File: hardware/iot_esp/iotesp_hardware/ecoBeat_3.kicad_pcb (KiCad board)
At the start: 2 copper layers, 67.6 x 58.6 mm, 8 parts, among them J1 Test, P1 CONN_02X05, U1 WeMos_mini

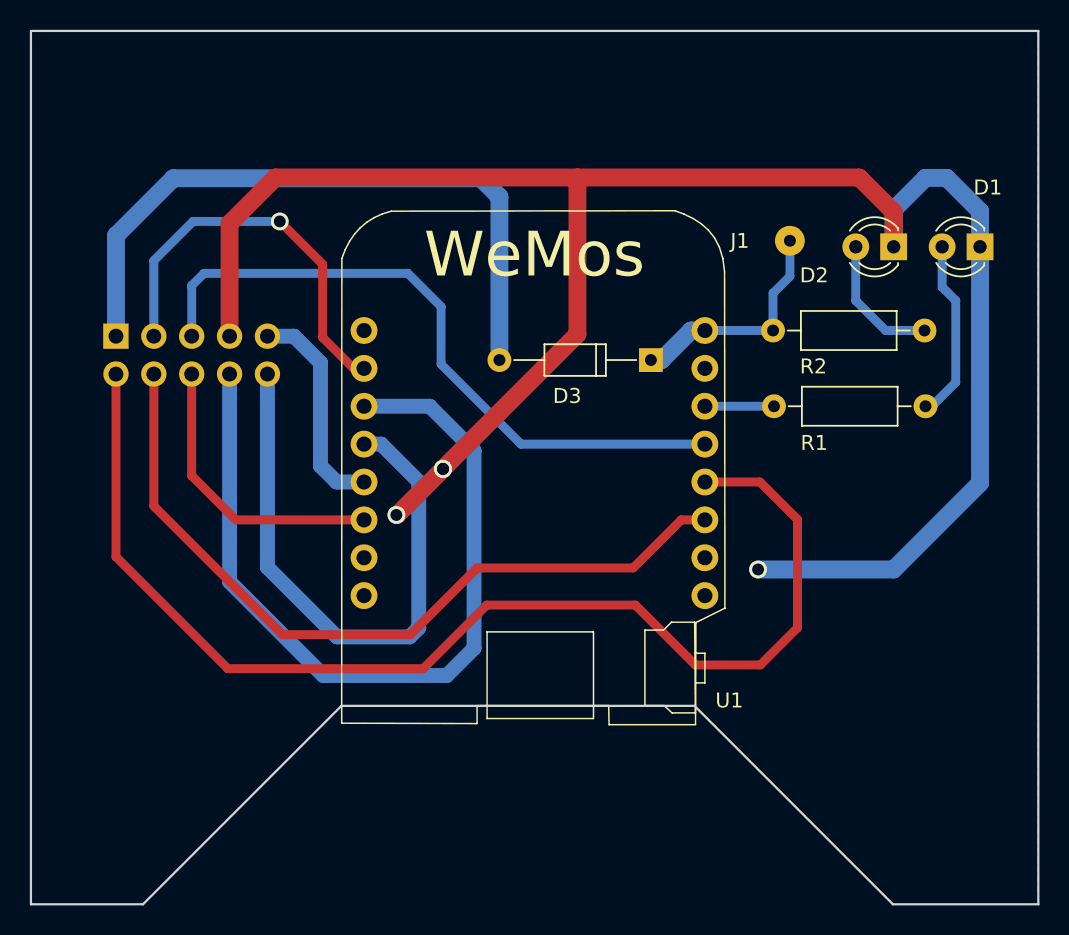
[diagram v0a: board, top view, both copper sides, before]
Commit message: PCB iot_esp12 v2 enviada a fabricar
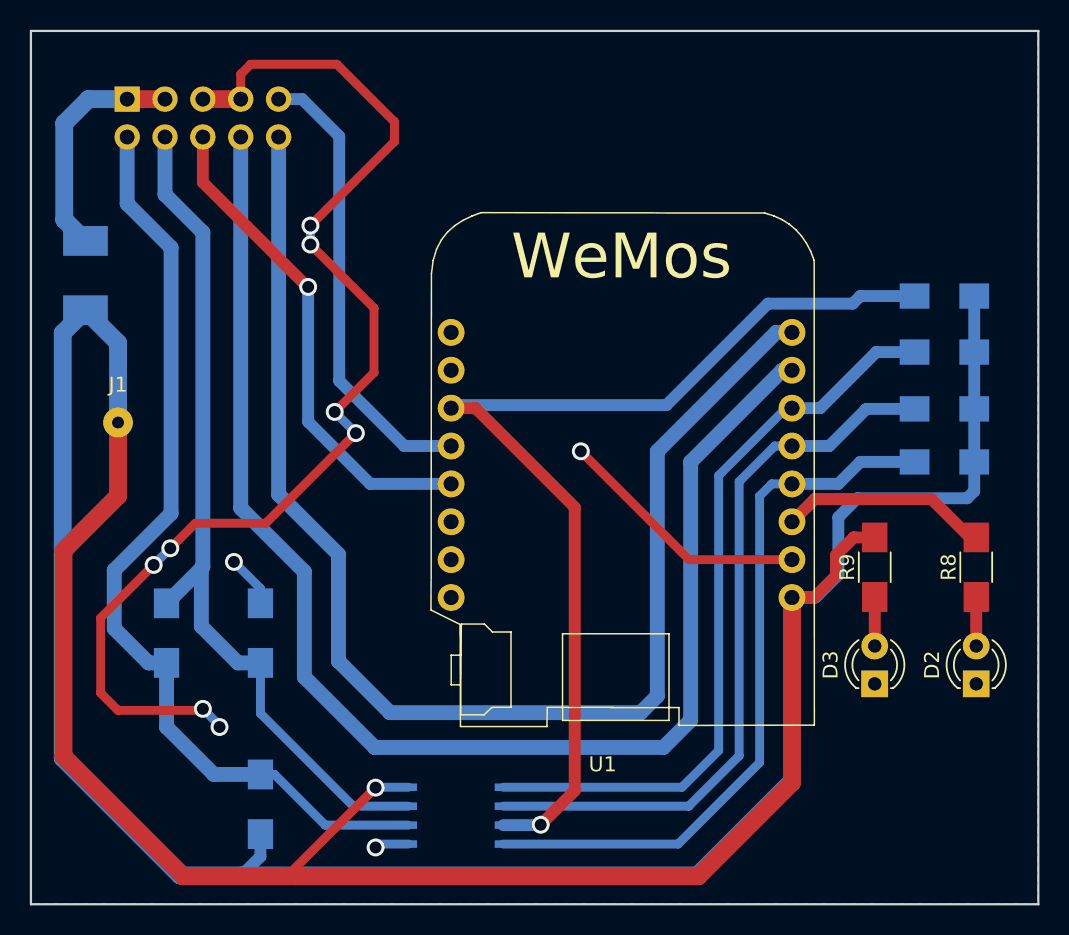
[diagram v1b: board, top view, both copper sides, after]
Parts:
- added R3: 10K, Resistors_SMD:R_1206_HandSoldering, B.Cu at (106.3, 49.1)
- added R4: 10K, Resistors_SMD:R_1206_HandSoldering, B.Cu at (106.3, 60.2)
- added R5: 20K, Resistors_SMD:R_1206_HandSoldering, B.Cu at (60.5, 83.2)
- added R6: 20K, Resistors_SMD:R_1206_HandSoldering, B.Cu at (60.5, 71.7)
- added R7: 120, Resistors_SMD:R_1206_HandSoldering, B.Cu at (54.2, 71.7)
- added R8: 220, Resistors_SMD:R_1206_HandSoldering, F.Cu at (108.5, 67.3)
- added R9: 220, Resistors_SMD:R_1206_HandSoldering, F.Cu at (101.7, 67.3)
- added U2: MAX_485, SMD_Packages:SOIC-8-N, B.Cu at (73.6, 84.0)
- D1: value LED -> Schottky; footprint LEDs:LED_D3.0mm -> Diodes_SMD:D_2114; moved to B.Cu
- D3: value Schottky -> LED; footprint Diodes_THT:D_DO-35_SOD27_P10.16mm_Horizontal -> LEDs:LED_D3.0mm
- R1, R2: value 220 -> 10K; footprint Resistors_THT:R_Axial_DIN0207_L6.3mm_D2.5mm_P10.16mm_Horizontal -> Resistors_SMD:R_1206_HandSoldering; moved to B.Cu
- U1: footprint wemos_d1_mini:D1_mini_board -> libreria_huellas_proyecto:D1_mini_board_oscar
- moved D1 60.0 mm to (48.7, 47.8), turned to 90 degrees
- moved J1 46.7 mm to (50.9, 57.6)
- moved D2 29.8 mm to (108.5, 75.1), turned to 90 degrees
- moved D3 26.4 mm to (101.7, 75.1), turned to 90 degrees
- moved P1 15.9 mm to (51.5, 35.9)
- moved U1 6.67 mm to (85.2, 59.6)
- moved R2 5.42 mm to (106.3, 56.7), turned to 0 degrees
- moved R1 3.85 mm to (106.3, 52.9), turned to 0 degrees
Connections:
- net /sck renamed /esp_d5
- D1 pad 1: GND -> /vin_5v
- D1 pad 2: Net-(D1-Pad2) -> VCC
- D3 pad 1: /vin_5v -> GND
- D3 pad 2: /vcc_5v -> Net-(D3-Pad2)
- P1 pad 1: /vcc_5v -> VCC
- P1 pad 10: /miso -> /esp_tx
- P1 pad 2: /esp_d2 -> /mb_a
- P1 pad 3: /esp_d8 -> VCC
- P1 pad 4: /esp_d1 -> /mb_b
- P1 pad 5: /esp_d3 -> GND
- P1 pad 6: /esp_d0 -> /esp_d6
- P1 pad 8: /mosi -> /esp_rx
- R1 pad 1: Net-(D1-Pad2) -> /esp_rx2
- R1 pad 2: /esp_d4 -> /vin_5v
- R2 pad 1: Net-(D2-Pad2) -> /esp_d2
- U1 pad 12: /esp_d3 -> /esp_tx2
- U1 pad 14: /esp_d1 -> /esp_rx2
- U1 pad 15: Net-(U1-Pad15) -> /esp_rx
- U1 pad 16: Net-(U1-Pad16) -> /esp_tx
- U1 pad 5: /miso -> /esp_d6
- U1 pad 6: /mosi -> Net-(U1-Pad6)
- U1 pad 7: /esp_d8 -> Net-(U1-Pad7)
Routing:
- net /vin_5v: track 15.5 -> 250.1 mm, vias 0 -> 1
- net /esp_rx: track 0.00 -> 93.3 mm
- net /esp_tx: track 0.00 -> 88.8 mm
- net /mb_a: track 0.00 -> 63.5 mm
- net /mb_b: track 0.00 -> 58.2 mm
- net /mosi: track 55.6 -> 0.00 mm
- net /esp_d1: track 52.6 -> 0.00 mm
- net /esp_rx2: track 0.00 -> 50.5 mm
- net /esp_d0: track 19.6 -> 70.0 mm, vias 0 -> 1
- net /esp_tx2: track 0.00 -> 48.7 mm
- net /esp_d3: track 45.9 -> 0.00 mm
- net /vcc_5v: track 45.8 -> 0.00 mm
- net /miso: track 39.8 -> 0.00 mm
- net /esp_d6: track 0.00 -> 33.4 mm, vias 0 -> 1
- net /esp_d2: track 80.0 -> 49.4 mm
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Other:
- outline, holes or cut-outs redrawn
